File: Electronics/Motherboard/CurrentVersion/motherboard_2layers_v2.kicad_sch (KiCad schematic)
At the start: 87 parts, among them J1 Conn_02x10_Odd_Even, J2 SSD1306, J3 USB_C_Receptacle_USB2.0_16P, J4 Micro_SD_Card_Det2, J5 Encoder, Q1 FDMS86202, Q2 FDMS86202, Q3 AO3400A, Q4 AO3400A, Q5 AO3400A, SW1 SW_Push, U1 TMC2209_SilentStepStick, U2 TMC2209_SilentStepStick, U3 LY1576HVS-5, U4 TMC2209_SilentStepStick, U5 TMC2209_SilentStepStick, U6 STZ12F405RGTx, U7 AMS1117-3.3, U8 AW9523B, U9 USBLC6-2SC6

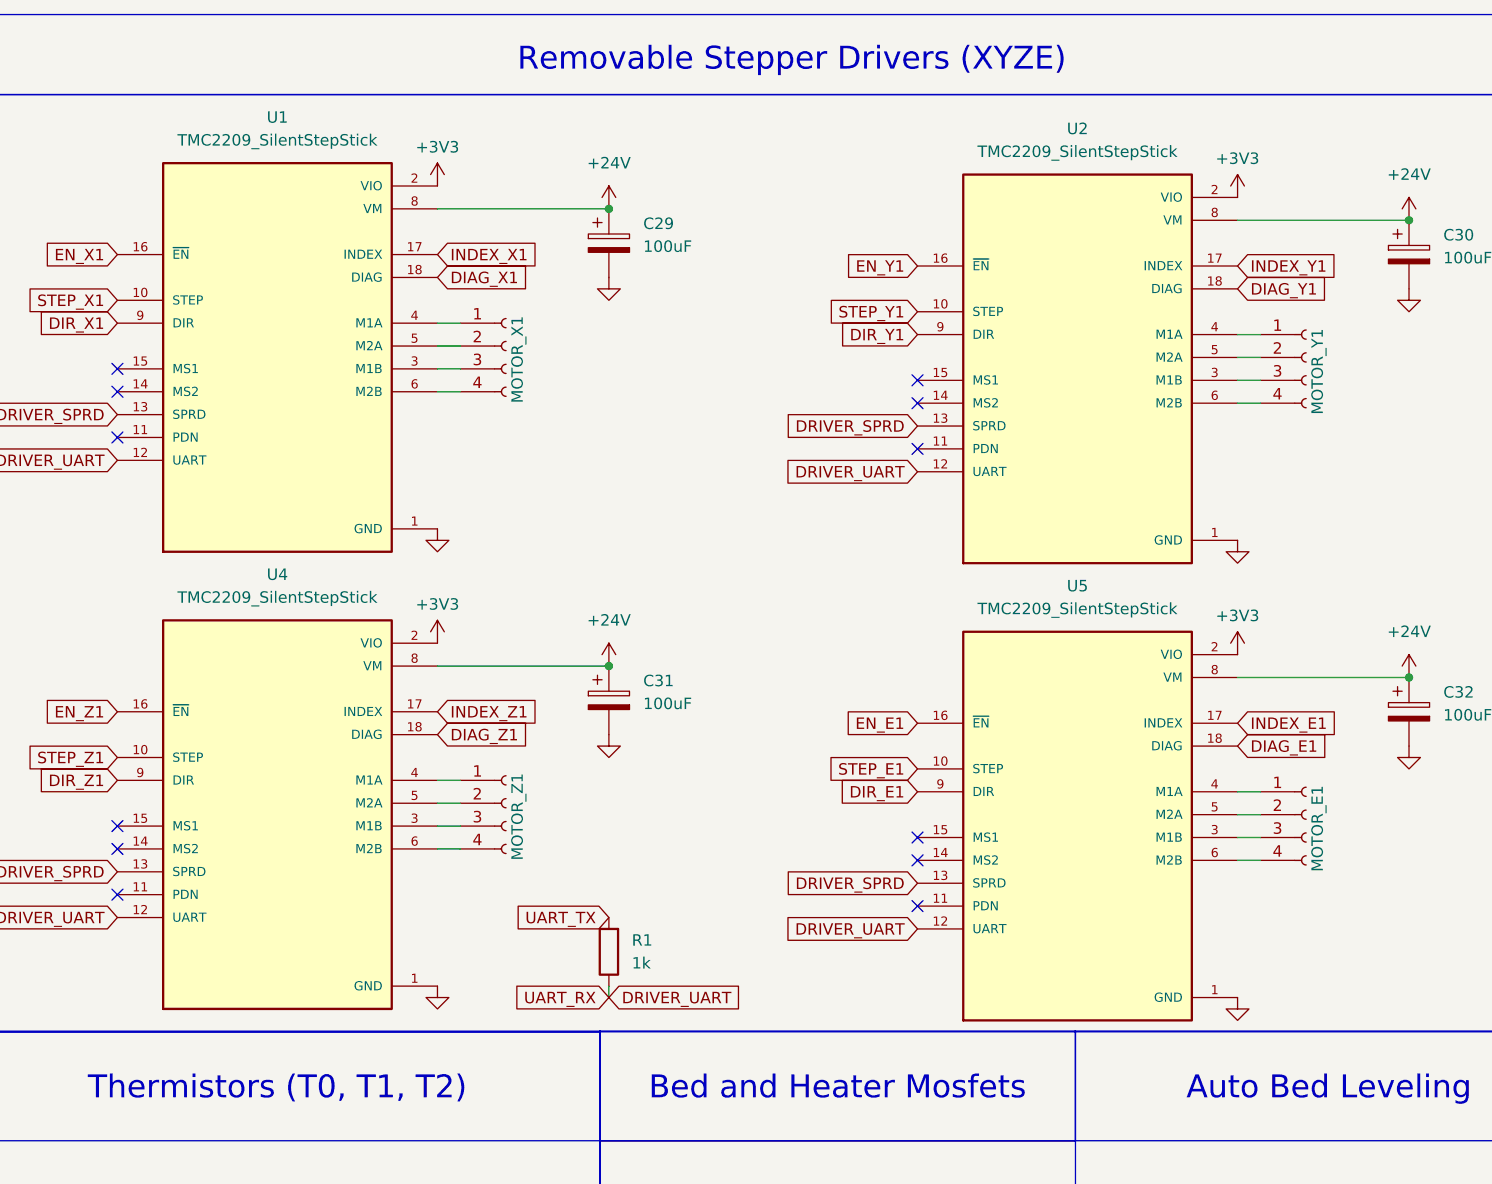
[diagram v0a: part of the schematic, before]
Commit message: aaaaaa many new thingies
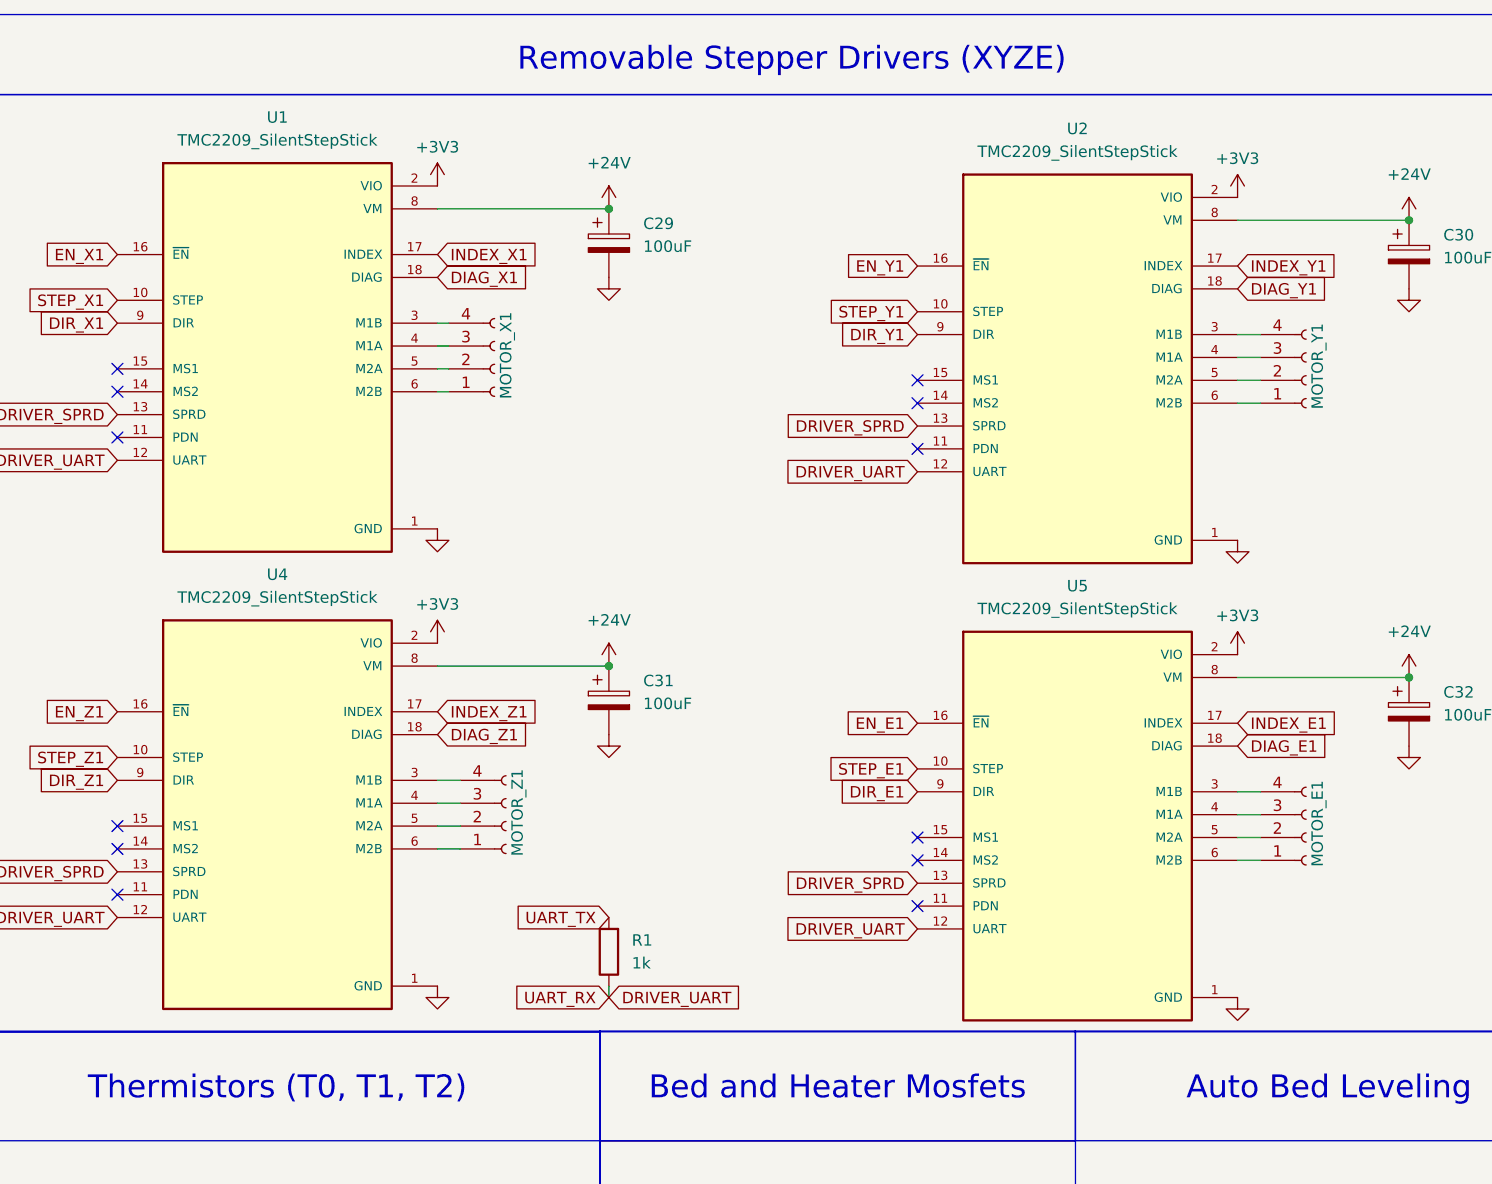
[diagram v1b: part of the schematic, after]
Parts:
- C10, C11, C12, C13, C14, C15, C16, C17, C18, C3, C4, C5, C6, C7, C8, C9: footprint Capacitor_SMD:C_0402_1005Metric -> Capacitor_SMD:C_0201_0603Metric; Part # TCC0402X7R104K160AT -> GRM033R61A104KE15D
- FAN1, FAN2, FAN3: footprint ad-hoc:ScrewTerminal-2pin-MKDS_1_2-3_5 -> Connector_JST:JST_XH_B2B-XH-A_1x02_P2.50mm_Vertical
- U8: footprint Package_DFN_QFN:QFN-24-1EP_4x4mm_P0.5mm_EP2.7x2.7mm_ThermalVias -> Package_DFN_QFN:QFN-24-1EP_4x4mm_P0.5mm_EP2.7x2.7mm
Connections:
- net at U5.3 (M1B): now also MOTOR_E1.4 (Pin_4); no longer MOTOR_E1.3 (Pin_3)
- net at U5.4 (M1A): now also MOTOR_E1.3 (Pin_3); no longer MOTOR_E1.1 (Pin_1)
- net at U5.6 (M2B): now also MOTOR_E1.1 (Pin_1); no longer MOTOR_E1.4 (Pin_4)
- net at U2.3 (M1B): now also MOTOR_Y1.4 (Pin_4); no longer MOTOR_Y1.3 (Pin_3)
- net at U2.4 (M1A): now also MOTOR_Y1.3 (Pin_3); no longer MOTOR_Y1.1 (Pin_1)
- net at U2.6 (M2B): now also MOTOR_Y1.1 (Pin_1); no longer MOTOR_Y1.4 (Pin_4)
- net at U4.3 (M1B): now also MOTOR_Z1.4 (Pin_4); no longer MOTOR_Z1.3 (Pin_3)
- net at U4.4 (M1A): now also MOTOR_Z1.3 (Pin_3); no longer MOTOR_Z1.1 (Pin_1)
- net at U4.6 (M2B): now also MOTOR_Z1.1 (Pin_1); no longer MOTOR_Z1.4 (Pin_4)
- net at MOTOR_X1.1 (Pin_1): now also U1.6 (M2B); no longer U1.4 (M1A)
- net at MOTOR_X1.3 (Pin_3): now also U1.4 (M1A); no longer U1.3 (M1B)
- net at MOTOR_X1.4 (Pin_4): now also U1.3 (M1B); no longer U1.6 (M2B)
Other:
- moved on the sheet: MOTOR_X1
